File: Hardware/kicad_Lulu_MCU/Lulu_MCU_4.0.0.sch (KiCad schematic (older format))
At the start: 13 parts, among them J1 Conn_01x03_Female, Q1 Q_NMOS_GSD, T1 Q_NPN_BEC, U1 ATtiny10-TS

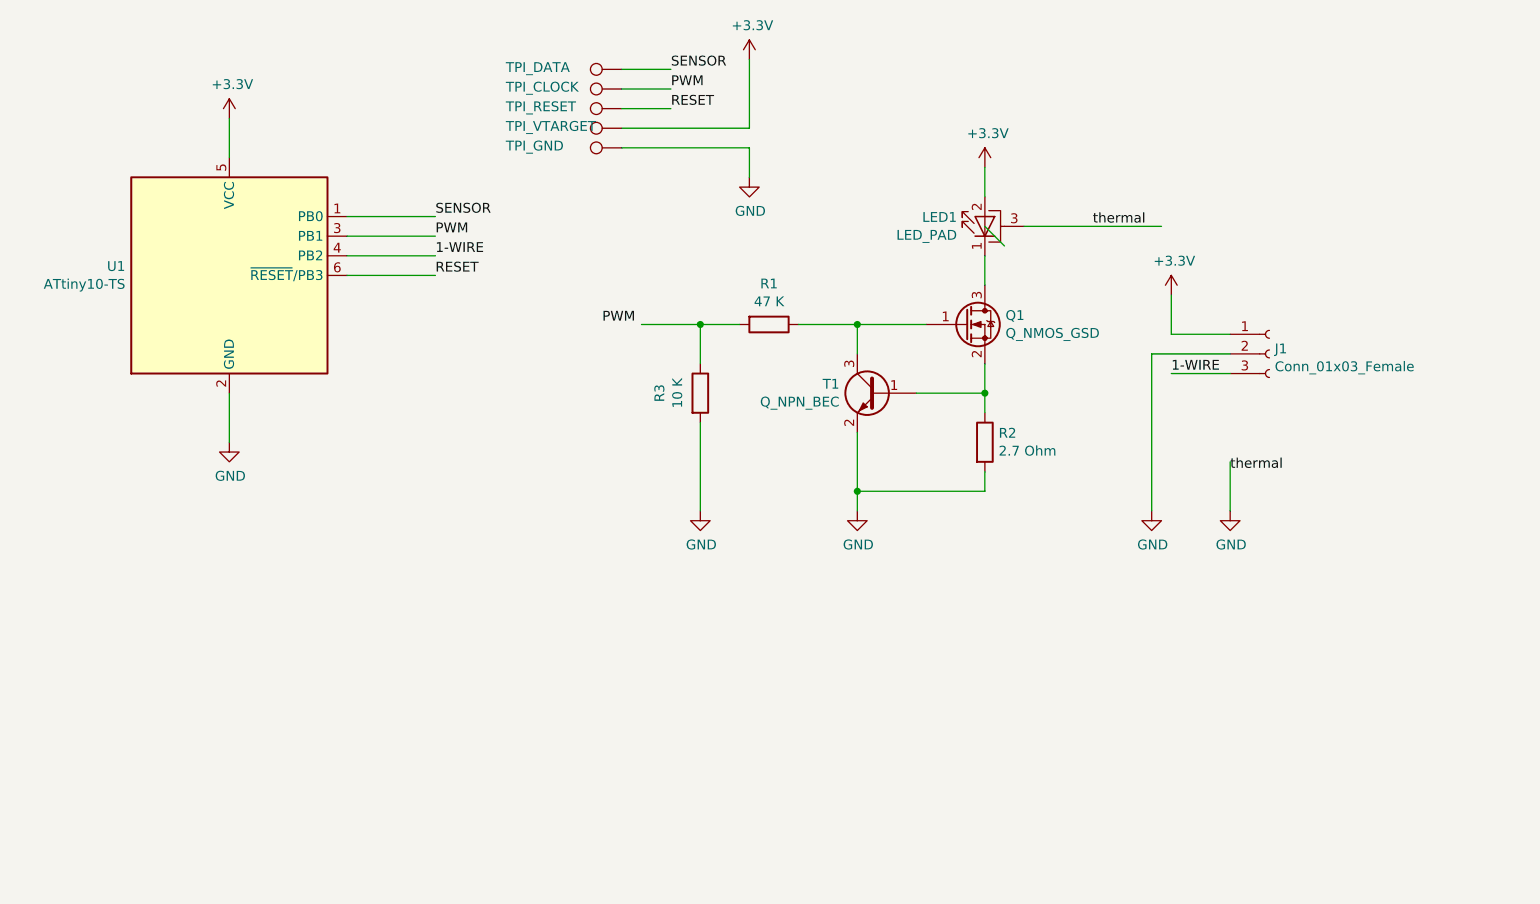
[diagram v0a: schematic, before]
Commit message: Under routing
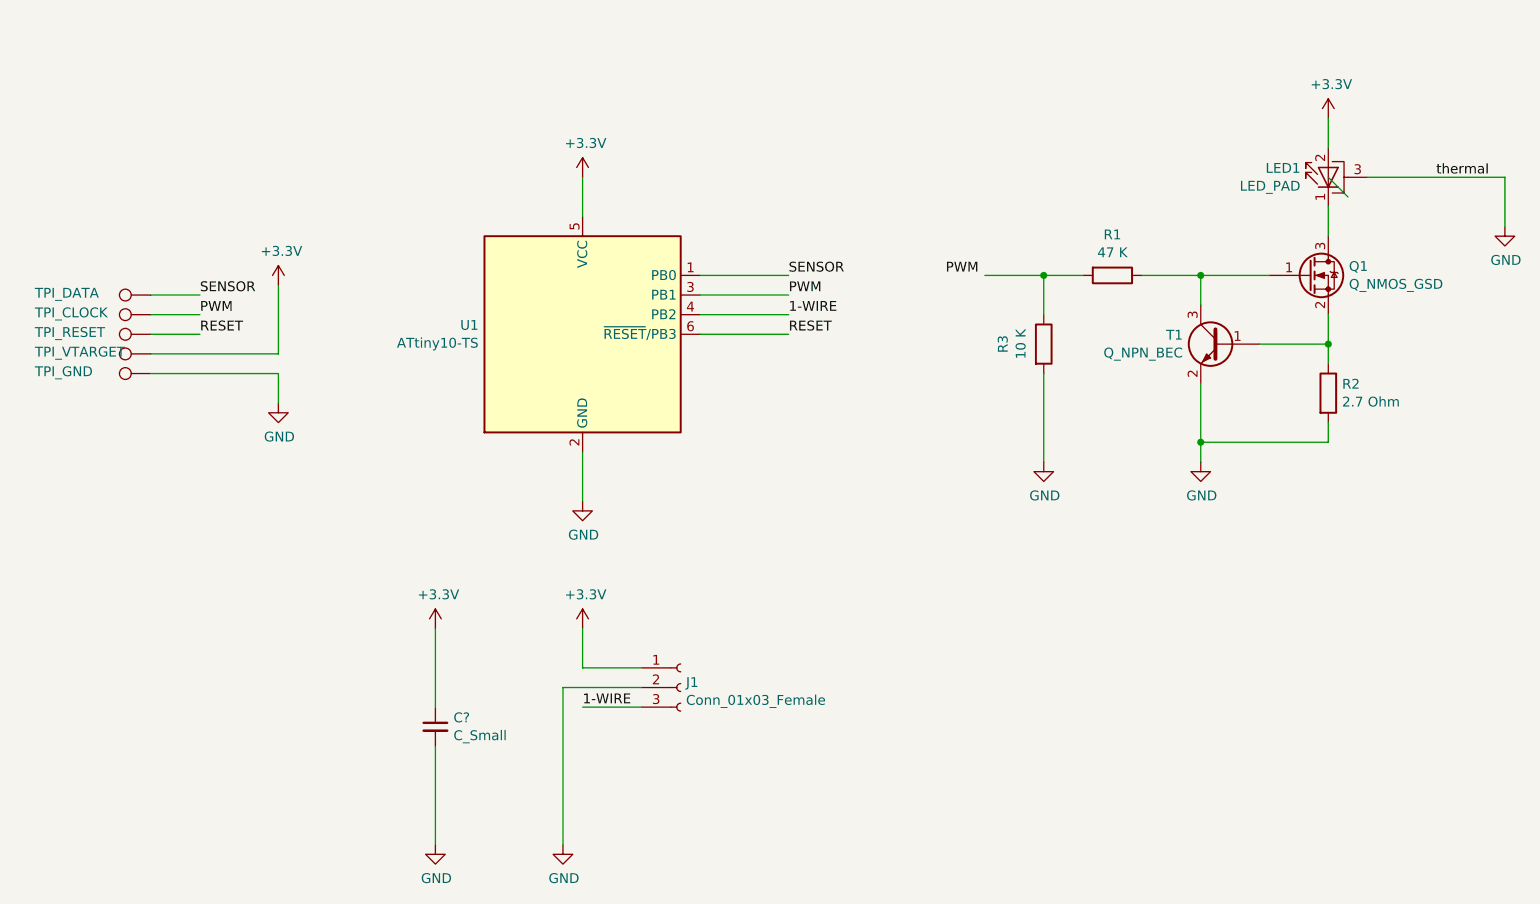
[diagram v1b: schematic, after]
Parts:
- added C?: C_Small, symbol Device:C_Small
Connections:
- wire segments 36 -> 38
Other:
- moved on the sheet: J1, LED1, Q1, R1, R2, R3, T1, U1
